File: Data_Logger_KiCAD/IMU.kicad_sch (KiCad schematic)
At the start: 9 parts, among them U1 LSM6DSO32TR, U3 ADXL375, U5 BMI088

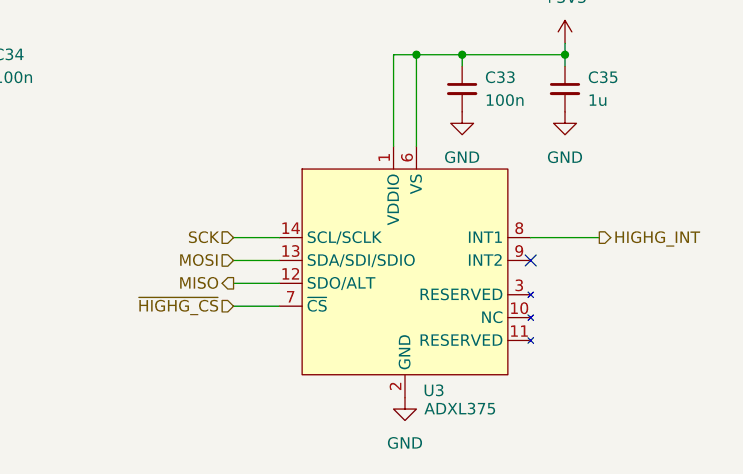
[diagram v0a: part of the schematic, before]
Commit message: partial MCU layout
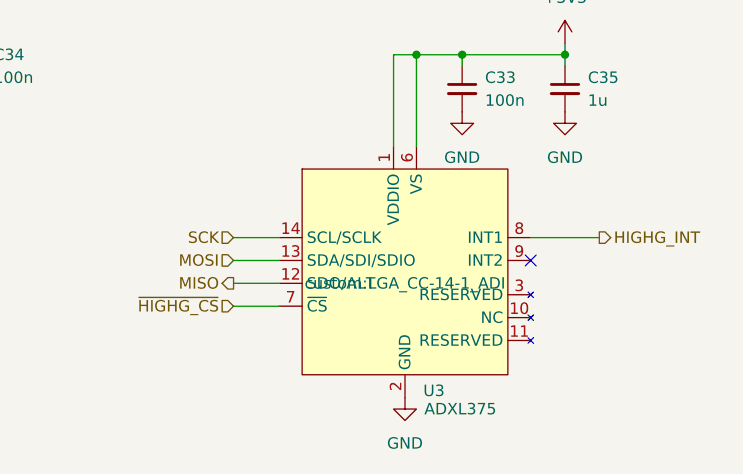
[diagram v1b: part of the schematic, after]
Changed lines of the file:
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@@
 					(size 1.27 1.27)
 				)
-				(hide yes)
 			)
 		)
